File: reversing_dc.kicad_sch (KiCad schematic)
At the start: 23 parts, among them IC1 IFX007TAUMA1, IC2 IFX007TAUMA1

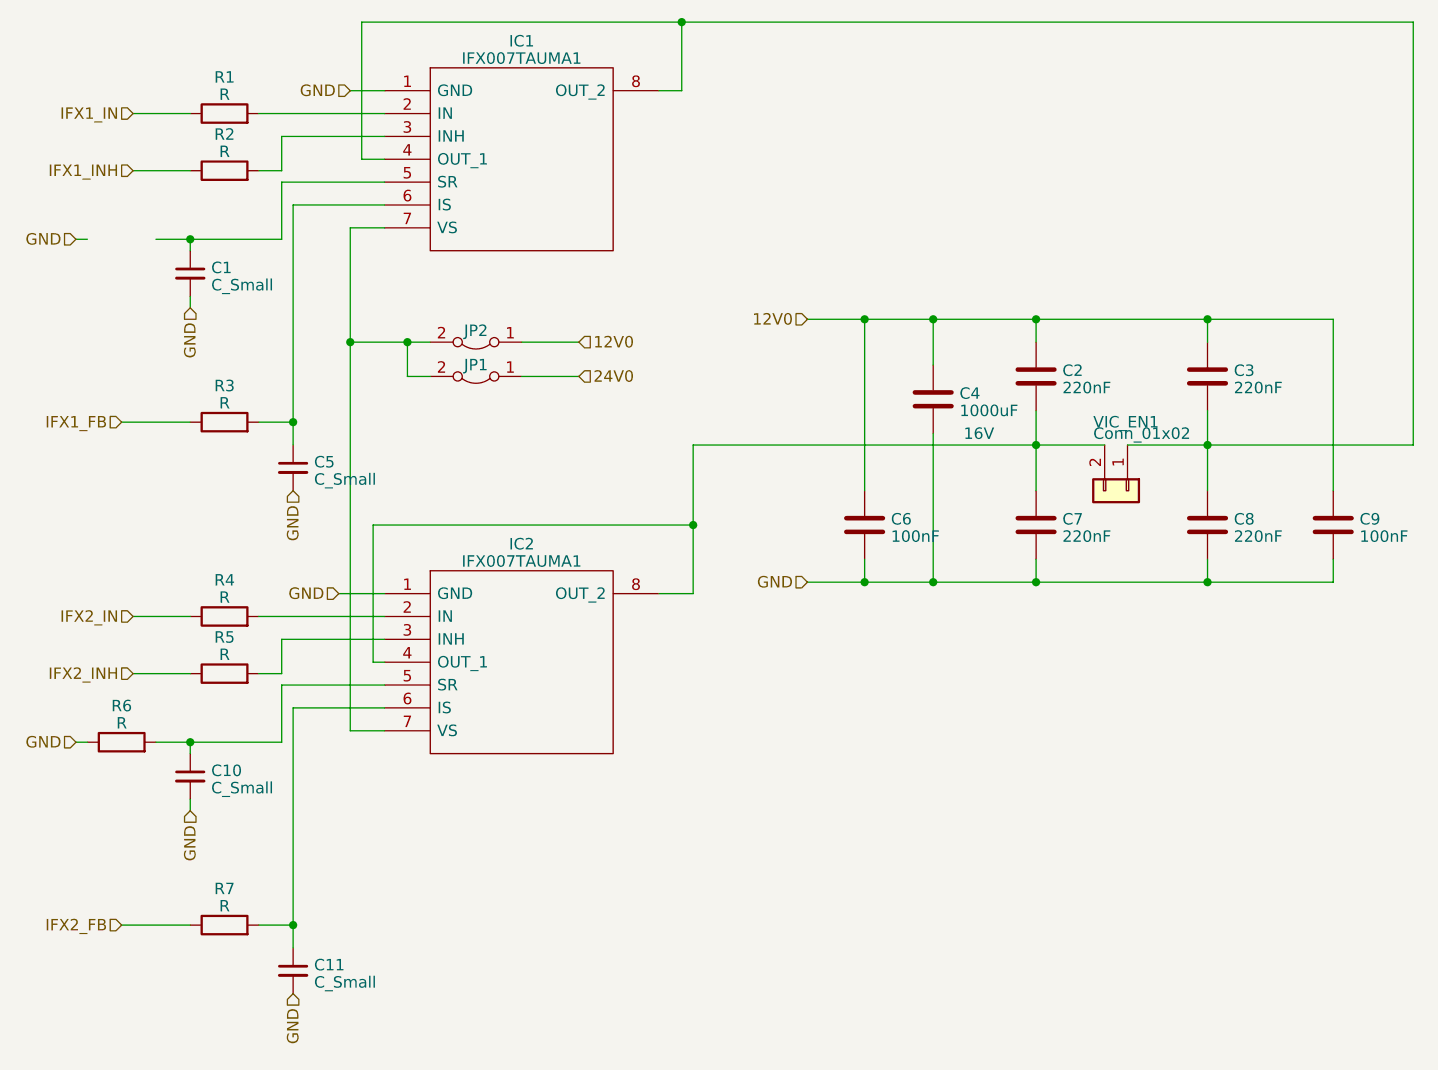
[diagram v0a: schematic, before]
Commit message: placing
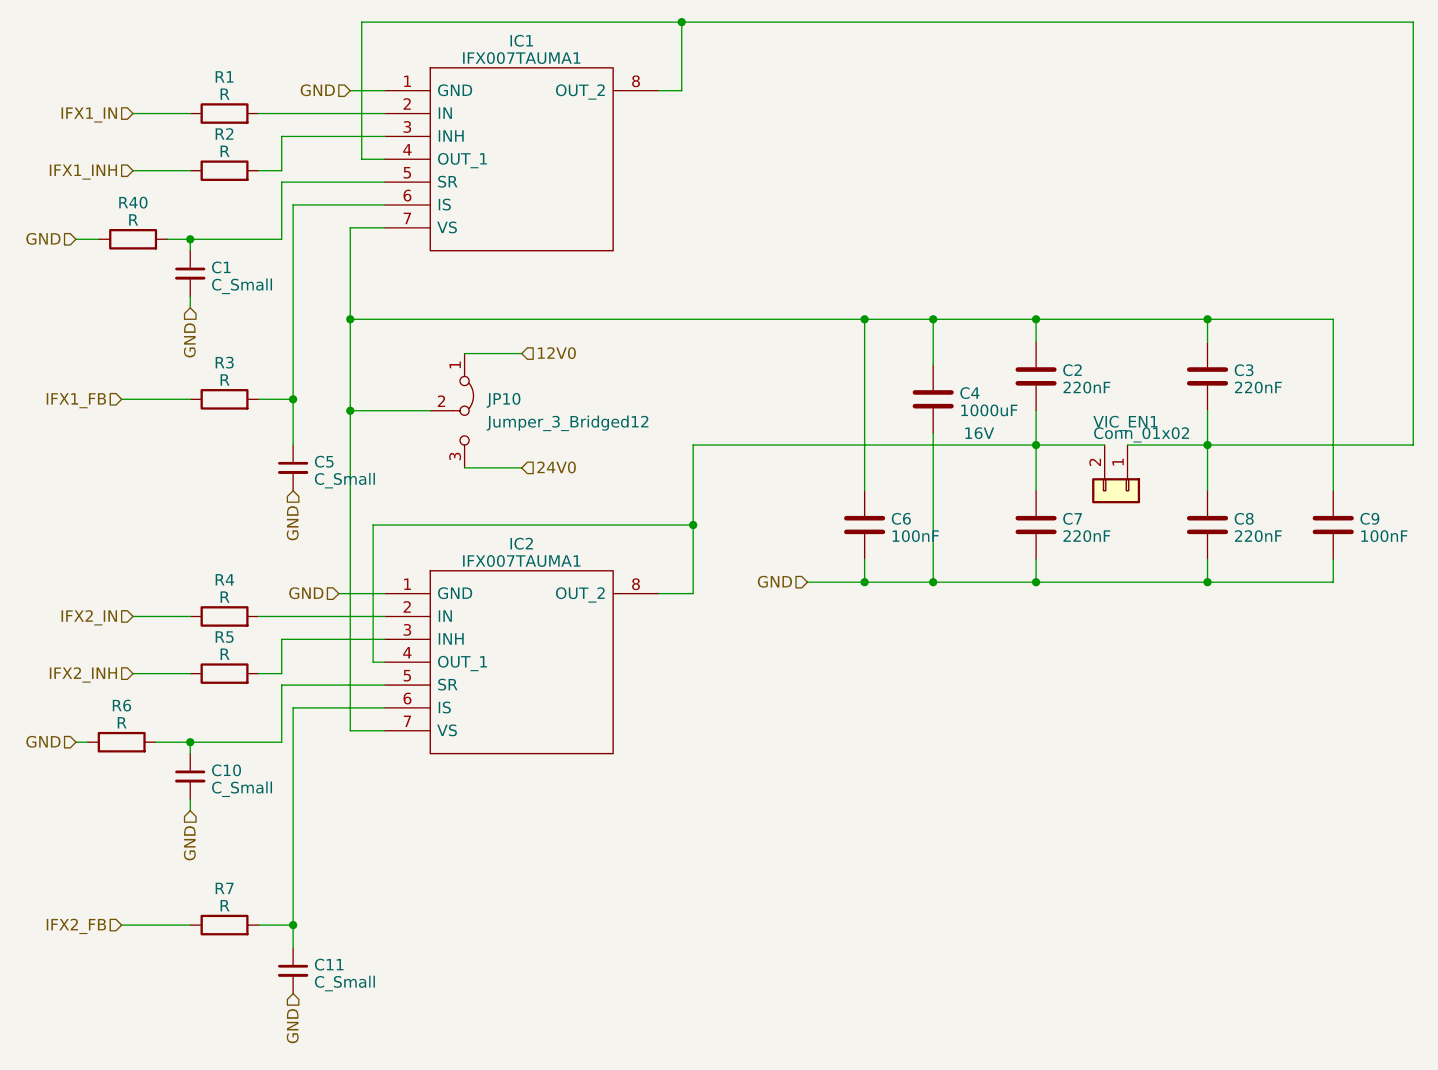
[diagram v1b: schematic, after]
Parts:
- removed JP1, JP2: Jumper_2_Bridged, symbol Jumper:Jumper_2_Bridged
- added JP10: Jumper_3_Bridged12, Connector_PinHeader_2.54mm:PinHeader_1x03_P2.54mm_Vertical, symbol Jumper:Jumper_3_Bridged12
- added R40: R, Resistor_SMD:R_0201_0603Metric_Pad0.64x0.40mm_HandSolder, symbol Device:R
- C1, C10, C11, C5, C6, C9: footprint (none) -> Capacitor_SMD:C_0603_1608Metric_Pad1.08x0.95mm_HandSolder
- C2, C3, C7, C8: footprint (none) -> Capacitor_SMD:C_0805_2012Metric_Pad1.18x1.45mm_HandSolder
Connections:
- net 12V0: now also JP10.1 (A); no longer C2.1, C3.1, C4.1, C6.1, C9.1
- net 24V0: now also JP10.3 (B)
- net GND: now also R40.1
- net at C1.1, IC1.5 (SR): now also R40.2
- net at IC1.7 (VS), IC2.7 (VS): now also C2.1, C3.1, C4.1, C6.1, C9.1, JP10.2 (C)
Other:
- moved on the sheet: R3

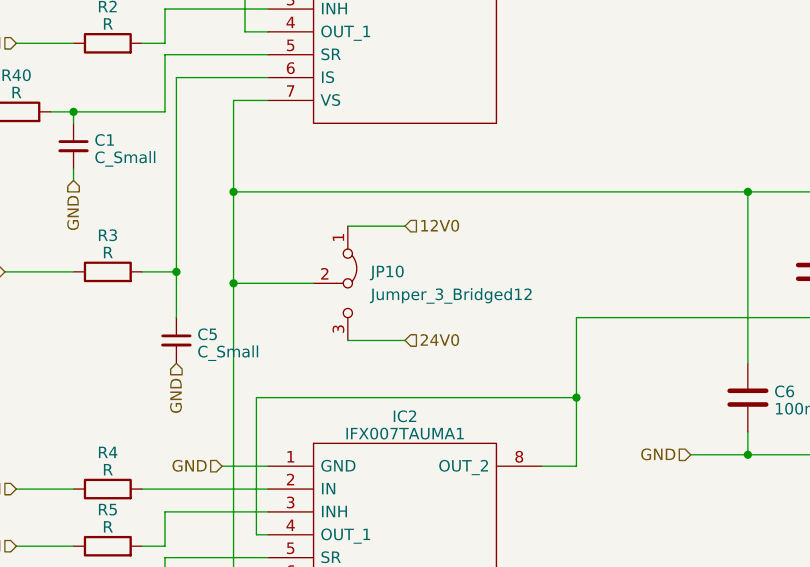
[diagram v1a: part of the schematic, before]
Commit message: gsdfg
dyfg
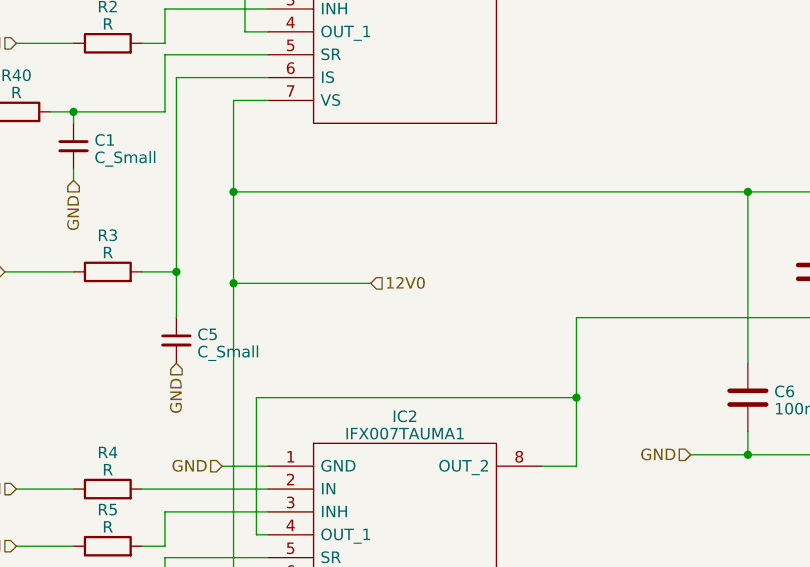
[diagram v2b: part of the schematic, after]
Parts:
- removed JP10: Jumper_3_Bridged12, Connector_PinHeader_2.54mm:PinHeader_1x03_P2.54mm_Vertical, symbol Jumper:Jumper_3_Bridged12
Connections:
- net 12V0: now also C2.1, C3.1, C4.1, C6.1, C9.1, IC1.7 (VS), IC2.7 (VS)
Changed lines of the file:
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@@
-    (stroke (width 0) (type default))
-  )
-  (wire (pts (xy 177.8 97.79) (xy 171.45 97.79))
     (stroke (width 0) (type default))
   )
@@
     (stroke (width 0) (type default))
   )
-  (wire (pts (xy 177.8 85.09) (xy 171.45 85.09))
-    (stroke (width 0) (type default))
-  )
   (wire (pts (xy 133.35 90.17) (xy 140.97 90.17))
     (stroke (width 0) (type default))
@@
     (stroke (width 0) (type default))
   )
-  (wire (pts (xy 158.75 91.44) (xy 167.64 91.44))
+  (wire (pts (xy 158.75 91.44) (xy 173.99 91.44))
     (stroke (width 0) (type default))
   )
@@
     (effects (font (size 1.27 1.27)) (justify right))
   )
-  (hierarchical_label "12V0" (shape input) (at 177.8 85.09 0) (fields_autoplaced)
+  (hierarchical_label "12V0" (shape input) (at 173.99 91.44 0) (fields_autoplaced)
     (effects (font (size 1.27 1.27)) (justify left))
   )
@@
   (hierarchical_label "IFX1_FB" (shape input) (at 133.35 90.17 180) (fields_autoplaced)
     (effects (font (size 1.27 1.27)) (justify right))
-  )
-  (hierarchical_label "24V0" (shape input) (at 177.8 97.79 0) (fields_autoplaced)
-    (effects (font (size 1.27 1.27)) (justify left))
   )
   (hierarchical_label "GND" (shape input) (at 128.27 72.39 180) (fields_autoplaced)
@@
         )
       )
-    )
-  )
-  (symbol (lib_id "Jumper:Jumper_3_Bridged12") (at 171.45 91.44 270) (unit 1)
-    (in_bom yes) (on_board yes) (dnp no) (fields_autoplaced)
-    (property "Reference" "JP10" (at 173.99 90.17 90)
-      (effects (font (size 1.27 1.27)) (justify left))
-    )
-    (property "Value" "Jumper_3_Bridged12" (at 173.99 92.71 90)
-      (effects (font (size 1.27 1.27)) (justify left))
-    )
-    (property "Footprint" "Connector_PinHeader_2.54mm:PinHeader_1x03_P2.54mm_Vertical" (at 171.45 91.44 0)
-      (effects (font (size 1.27 1.27)) hide)
-    )
-    (property "Datasheet" "~" (at 171.45 91.44 0)
-      (effects (font (size 1.27 1.27)) hide)
-    )
-    (pin "1")
-    (pin "2")
-    (pin "3")
-    (instances
-      (project "rollo control"
-        (path "/7fd4875b-e2b3-49e9-a377-320ee6c6aef7/42cd8867-79f6-4c26-8217-42f6d2cc80dc"
-          (reference "JP10") (unit 1)
-        )
-        (path "/7fd4875b-e2b3-49e9-a377-320ee6c6aef7/f84d4e41-04bc-49f0-bae3-d4cb51e0b9a0"
-          (reference "JP7") (unit 1)
-        )
-        (path "/7fd4875b-e2b3-49e9-a377-320ee6c6aef7/4e3087fc-fc79-4dc0-b9f3-dc50efd75935"
-          (reference "JP8") (unit 1)
-        )
-      )
